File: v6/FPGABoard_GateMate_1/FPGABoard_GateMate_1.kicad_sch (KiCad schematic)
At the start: 0 parts

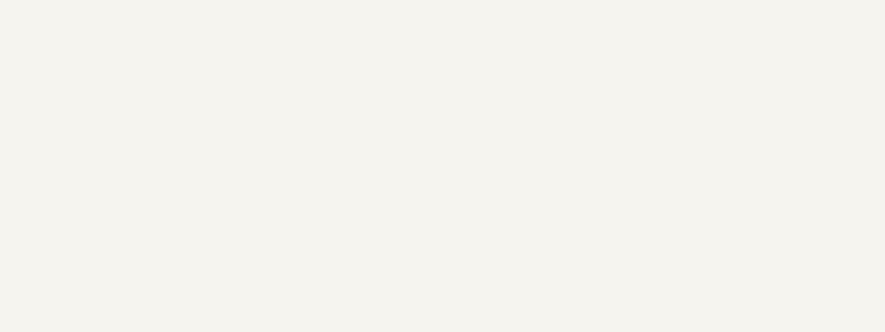
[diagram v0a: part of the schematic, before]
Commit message: First review of base module done
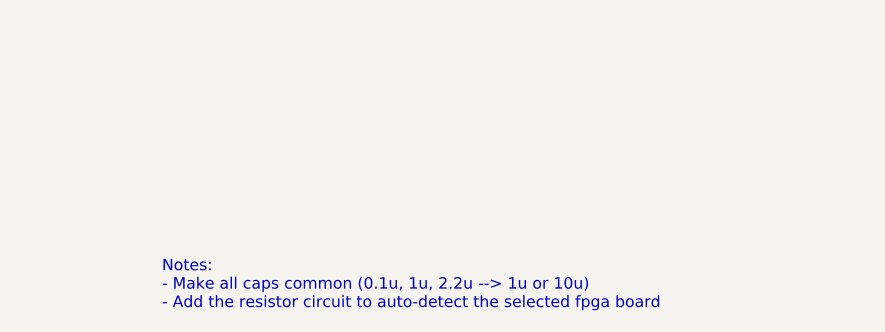
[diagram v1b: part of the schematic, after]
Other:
- note added: "Notes: - Make all caps common (0.1u, 1u, 2.2u --> 1u or 10u) - Add the resistor circuit to auto-detect the selected fpga board"
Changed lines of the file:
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@@
 	(generator_version "10.0")
 	(paper "A4")
+	(text "Notes:\n- Make all caps common (0.1u, 1u, 2.2u --> 1u or 10u)\n- Add the resistor circuit to auto-detect the selected fpga board"
+		(exclude_from_sim no)
+		(at 177.546 166.624 0)
+		(effects
+			(font
+				(size 1.27 1.27)
+			)
+			(justify left top)
+		)
+	)
 	(text "General: Add testpads for specific signals which will not be moved to other boards"
 		(exclude_from_sim no)
